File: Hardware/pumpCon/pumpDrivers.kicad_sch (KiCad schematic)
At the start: 50 parts, among them J10 Conn_01x02, J11 Conn_01x02, J12 Conn_01x05, J13 Conn_01x05, J14 Conn_01x05, J15 Conn_01x05, J16 Conn_01x05, J17 Conn_01x05, J18 Conn_01x05, J19 Conn_01x05, U10 74HC595, U11 ULN2003F12, U12 ULN2003F12, U13 ULN2003F12, U14 ULN2003F12, U15 74HC595, U16 74HC595, U17 ULN2003F12, U18 ULN2003F12, U19 ULN2003F12, U20 ULN2003F12, U7 DRV8231ADSGR, U8 DRV8231ADSGR, U9 74HC595

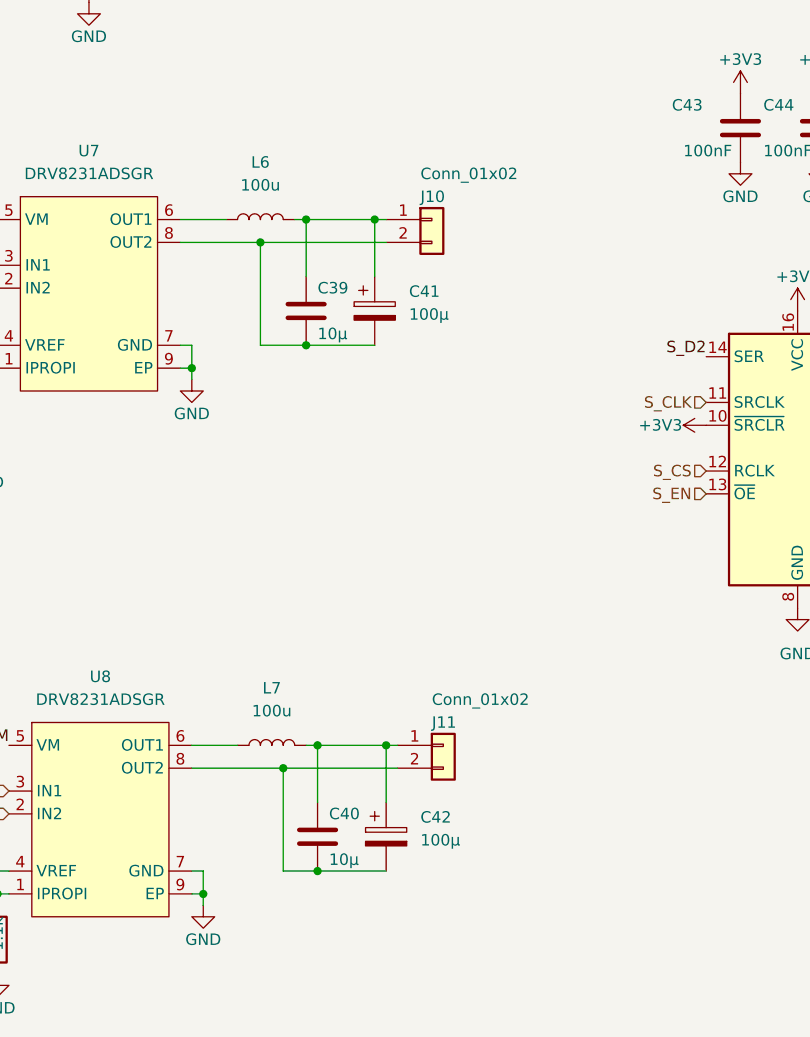
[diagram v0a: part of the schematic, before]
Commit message: pumpCon fully work now
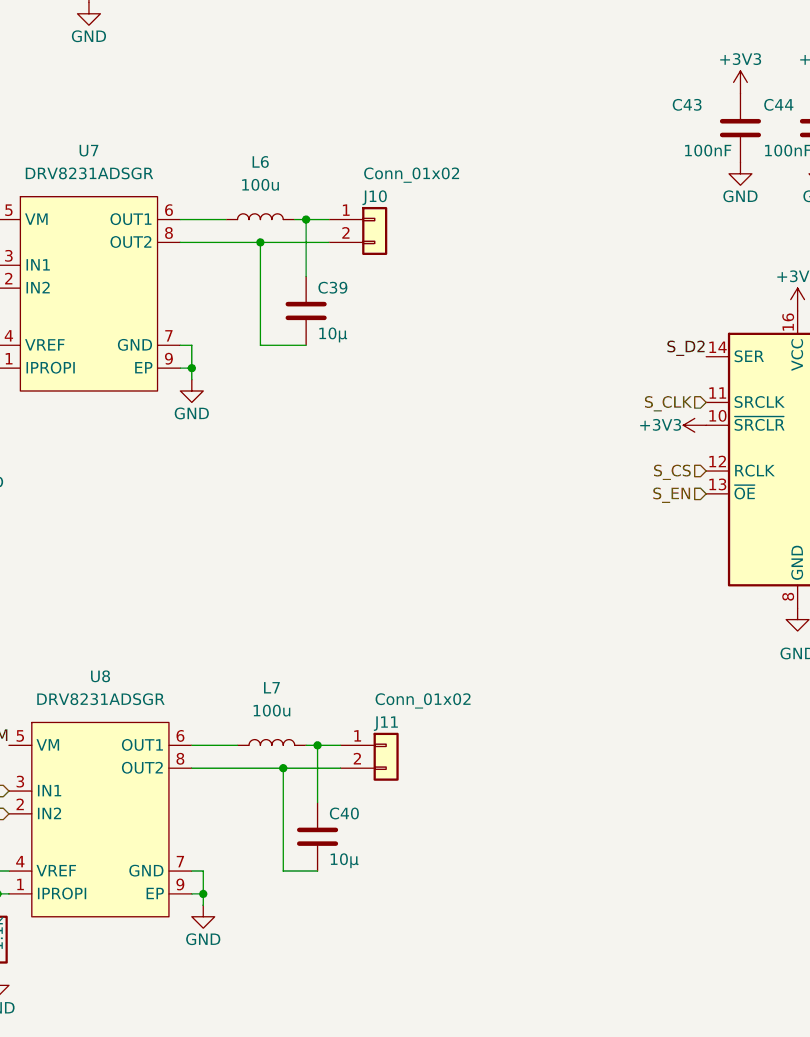
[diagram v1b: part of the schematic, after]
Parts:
- removed C41, C42: 100µ, Capacitor_THT:CP_Radial_D6.3mm_P2.50mm, symbol Device:C_Polarized
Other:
- moved on the sheet: J10, J11
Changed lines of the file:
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@@
 (kicad_sch (version 20211123) (generator eeschema)
   (paper "A4")
-  (junction (at 93.98 113.03) (diameter 0) (color 0 0 0 0)
-  )
   (junction (at 261.62 80.01) (diameter 0) (color 0 0 0 0)
   )
@@
   (junction (at 275.59 133.35) (diameter 0) (color 0 0 0 0)
   )
-  (junction (at 95.25 171.45) (diameter 0) (color 0 0 0 0)
-  )
   (junction (at 261.62 153.67) (diameter 0) (color 0 0 0 0)
   )
@@
   (junction (at 177.8 153.67) (diameter 0) (color 0 0 0 0)
   )
-  (junction (at 101.6 99.06) (diameter 0) (color 0 0 0 0)
-  )
   (junction (at 177.8 45.72) (diameter 0) (color 0 0 0 0)
   )
@@
   (junction (at 59.69 173.99) (diameter 0) (color 0 0 0 0)
   )
-  (junction (at 102.87 157.48) (diameter 0) (color 0 0 0 0)
-  )
   (junction (at 275.59 95.25) (diameter 0) (color 0 0 0 0)
   )
@@
     (stroke (width 0) (type default) (color 0 0 0 0))
   )
-  (wire (pts (xy 102.87 157.48) (xy 104.14 157.48))
-    (stroke (width 0) (type default) (color 0 0 0 0))
-  )
   (wire (pts (xy 158.75 72.39) (xy 158.75 55.88))
     (stroke (width 0) (type default) (color 0 0 0 0))
@@
     (stroke (width 0) (type default) (color 0 0 0 0))
   )
-  (wire (pts (xy 93.98 99.06) (xy 101.6 99.06))
+  (wire (pts (xy 93.98 99.06) (xy 96.52 99.06))
     (stroke (width 0) (type default) (color 0 0 0 0))
   )
@@
     (stroke (width 0) (type default) (color 0 0 0 0))
   )
-  (wire (pts (xy 102.87 163.83) (xy 102.87 157.48))
-    (stroke (width 0) (type default) (color 0 0 0 0))
-  )
   (wire (pts (xy 177.8 45.72) (xy 180.34 45.72))
     (stroke (width 0) (type default) (color 0 0 0 0))
@@
     (stroke (width 0) (type default) (color 0 0 0 0))
   )
-  (wire (pts (xy 95.25 171.45) (xy 102.87 171.45))
-    (stroke (width 0) (type default) (color 0 0 0 0))
-  )
   (wire (pts (xy 241.3 55.88) (xy 238.76 55.88))
     (stroke (width 0) (type default) (color 0 0 0 0))
@@
     (stroke (width 0) (type default) (color 0 0 0 0))
   )
-  (wire (pts (xy 102.87 101.6) (xy 88.9 101.6))
+  (wire (pts (xy 96.52 101.6) (xy 88.9 101.6))
     (stroke (width 0) (type default) (color 0 0 0 0))
   )
@@
     (stroke (width 0) (type default) (color 0 0 0 0))
   )
-  (wire (pts (xy 101.6 113.03) (xy 93.98 113.03))
-    (stroke (width 0) (type default) (color 0 0 0 0))
-  )
   (wire (pts (xy 95.25 163.83) (xy 95.25 157.48))
     (stroke (width 0) (type default) (color 0 0 0 0))
@@
     (stroke (width 0) (type default) (color 0 0 0 0))
   )
-  (wire (pts (xy 95.25 157.48) (xy 102.87 157.48))
+  (wire (pts (xy 95.25 157.48) (xy 97.79 157.48))
     (stroke (width 0) (type default) (color 0 0 0 0))
   )
@@
     (stroke (width 0) (type default) (color 0 0 0 0))
   )
-  (wire (pts (xy 91.44 160.02) (xy 104.14 160.02))
+  (wire (pts (xy 91.44 160.02) (xy 97.79 160.02))
     (stroke (width 0) (type default) (color 0 0 0 0))
   )
@@
     (stroke (width 0) (type default) (color 0 0 0 0))
   )
-  (wire (pts (xy 101.6 99.06) (xy 102.87 99.06))
-    (stroke (width 0) (type default) (color 0 0 0 0))
-  )
   (wire (pts (xy 242.57 114.3) (xy 242.57 100.33))
     (stroke (width 0) (type default) (color 0 0 0 0))
@@
   )
   (wire (pts (xy 242.57 146.05) (xy 252.73 146.05))
-    (stroke (width 0) (type default) (color 0 0 0 0))
-  )
-  (wire (pts (xy 101.6 105.41) (xy 101.6 99.06))
     (stroke (width 0) (type default) (color 0 0 0 0))
   )
@@
     (pin "1")
   )
-  (symbol (lib_id "Device:C_Polarized") (at 101.6 109.22 0) (unit 1)
-    (in_bom yes) (on_board yes) (fields_autoplaced)
-    (property "Reference" "C41" (id 0) (at 105.41 107.0609 0)
-      (effects (font (size 1.27 1.27)) (justify left))
-    )
-    (property "Value" "100µ" (id 1) (at 105.41 109.6009 0)
-      (effects (font (size 1.27 1.27)) (justify left))
-    )
-    (property "Footprint" "Capacitor_THT:CP_Radial_D6.3mm_P2.50mm" (id 2) (at 102.5652 113.03 0)
-      (effects (font (size 1.27 1.27)) hide)
-    )
-    (property "Datasheet" "~" (id 3) (at 101.6 109.22 0)
-      (effects (font (size 1.27 1.27)) hide)
-    )
-    (pin "1")
-    (pin "2")
-  )
   (symbol (lib_id "Device:C") (at 232.41 86.36 0) (unit 1)
     (in_bom yes) (on_board yes)
@@
     (pin "2")
   )
-  (symbol (lib_id "Connector_Generic:Conn_01x02") (at 109.22 157.48 0) (unit 1)
-    (in_bom yes) (on_board yes)
-    (property "Reference" "J11" (id 0) (at 107.95 154.94 0)
-      (effects (font (size 1.27 1.27)) (justify left))
-    )
-    (property "Value" "Conn_01x02" (id 1) (at 107.95 152.4 0)
-      (effects (font (size 1.27 1.27)) (justify left))
-    )
-    (property "Footprint" "Connector_Molex:Molex_KK-254_AE-6410-02A_1x02_P2.54mm_Vertical" (id 2) (at 109.22 157.48 0)
-      (effects (font (size 1.27 1.27)) hide)
-    )
-    (property "Datasheet" "~" (id 3) (at 109.22 157.48 0)
+  (symbol (lib_id "Connector_Generic:Conn_01x02") (at 102.87 157.48 0) (unit 1)
+    (in_bom yes) (on_board yes)
+    (property "Reference" "J11" (id 0) (at 101.6 154.94 0)
+      (effects (font (size 1.27 1.27)) (justify left))
+    )
+    (property "Value" "Conn_01x02" (id 1) (at 101.6 152.4 0)
+      (effects (font (size 1.27 1.27)) (justify left))
+    )
+    (property "Footprint" "Connector_Molex:Molex_KK-254_AE-6410-02A_1x02_P2.54mm_Vertical" (id 2) (at 102.87 157.48 0)
+      (effects (font (size 1.27 1.27)) hide)
+    )
+    (property "Datasheet" "~" (id 3) (at 102.87 157.48 0)
       (effects (font (size 1.27 1.27)) hide)
     )
@@
     (pin "5")
   )
-  (symbol (lib_id "Device:C_Polarized") (at 102.87 167.64 0) (unit 1)
-    (in_bom yes) (on_board yes) (fields_autoplaced)
-    (property "Reference" "C42" (id 0) (at 106.68 165.4809 0)
-      (effects (font (size 1.27 1.27)) (justify left))
-    )
-    (property "Value" "100µ" (id 1) (at 106.68 168.0209 0)
-      (effects (font (size 1.27 1.27)) (justify left))
-    )
-    (property "Footprint" "Capacitor_THT:CP_Radial_D6.3mm_P2.50mm" (id 2) (at 103.8352 171.45 0)
-      (effects (font (size 1.27 1.27)) hide)
-    )
-    (property "Datasheet" "~" (id 3) (at 102.87 167.64 0)
-      (effects (font (size 1.27 1.27)) hide)
-    )
-    (pin "1")
-    (pin "2")
-  )
   (symbol (lib_id "power:GND") (at 275.59 123.19 0) (unit 1)
     (in_bom yes) (on_board yes)
@@
     (pin "1")
   )
-  (symbol (lib_id "Connector_Generic:Conn_01x02") (at 107.95 99.06 0) (unit 1)
-    (in_bom yes) (on_board yes)
-    (property "Reference" "J10" (id 0) (at 106.68 96.52 0)
-      (effects (font (size 1.27 1.27)) (justify left))
-    )
-    (property "Value" "Conn_01x02" (id 1) (at 106.68 93.98 0)
-      (effects (font (size 1.27 1.27)) (justify left))
-    )
-    (property "Footprint" "Connector_Molex:Molex_KK-254_AE-6410-02A_1x02_P2.54mm_Vertical" (id 2) (at 107.95 99.06 0)
-      (effects (font (size 1.27 1.27)) hide)
-    )
-    (property "Datasheet" "~" (id 3) (at 107.95 99.06 0)
-      (effects (font (size 1.27 1.27)) hide)
-    )
+  (symbol (lib_id "Connector_Generic:Conn_01x02") (at 101.6 99.06 0) (unit 1)
+    (in_bom yes) (on_board yes)
+    (property "Reference" "J10" (id 0) (at 100.33 96.52 0)
+      (effects (font (size 1.27 1.27)) (justify left))
+    )
+    (property "Value" "Conn_01x02" (id 1) (at 100.33 93.98 0)
+      (effects (font (size 1.27 1.27)) (justify left))
+    )
+    (property "Footprint" "Connector_Molex:Molex_KK-254_AE-6410-02A_1x02_P2.54mm_Vertical" (id 2) (at 101.6 99.06 0)
+      (effects (font (size 1.27 1.27)) hide)
+    )
+    (property "Datasheet" "~" (id 3) (at 101.6 99.06 0)
+      (effects (font (size 1.27 1.27)) hide)
+    )
